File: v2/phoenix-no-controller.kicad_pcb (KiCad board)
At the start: 2 copper layers, 121.5 x 110.3 mm, 66 parts

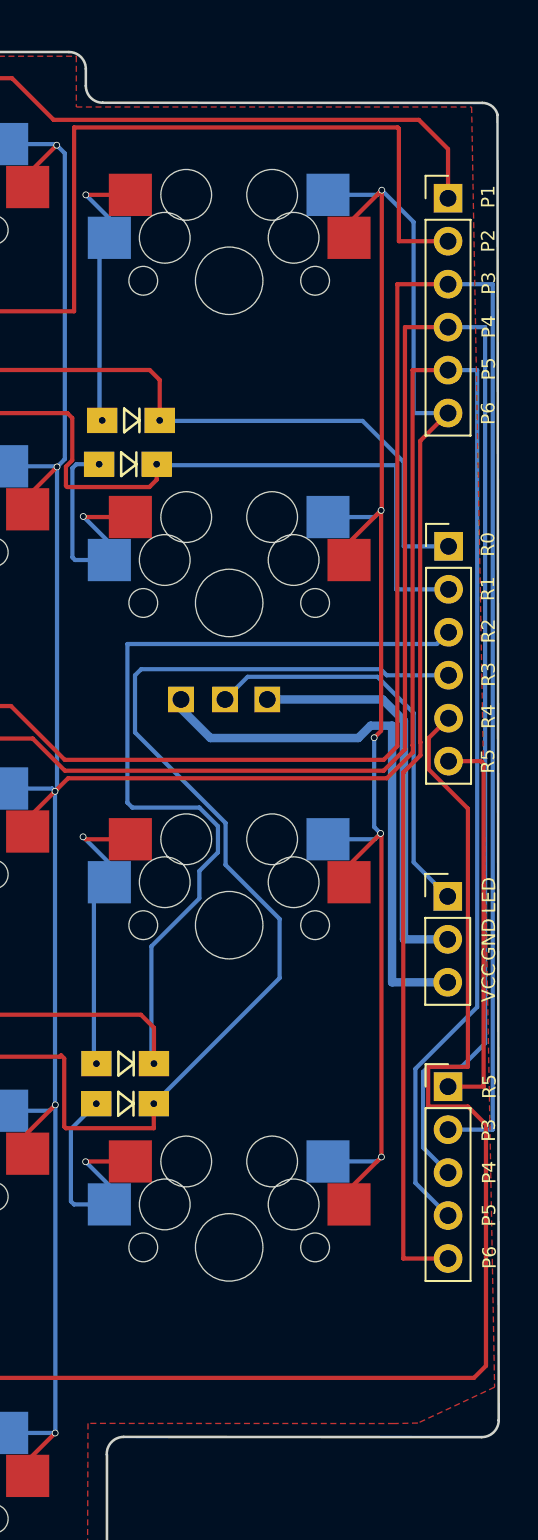
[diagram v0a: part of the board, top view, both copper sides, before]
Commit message: thumb
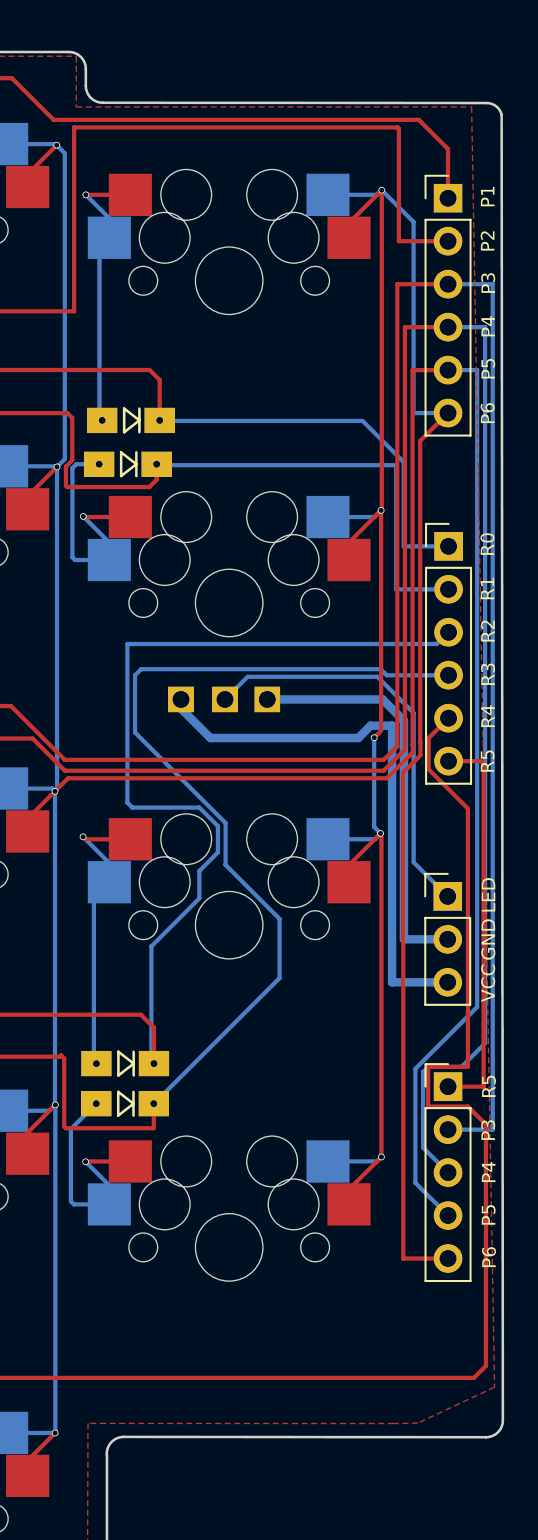
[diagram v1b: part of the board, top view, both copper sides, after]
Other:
- board size 121.5 x 110.3 mm -> 121.8 x 110.3 mm
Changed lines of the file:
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@@
   (gr_arc (start 209.0325 81.84981) (mid 208.325393 81.556917) (end 208.0325 80.84981)
     (stroke (width 0.15) (type solid)) (layer "Edge.Cuts"))
-  (gr_arc (start 250.47 84.86) (mid 251.03946 85.049183) (end 251.37 85.55)
+  (gr_arc (start 250.717102 84.867102) (mid 251.286538 85.056304) (end 251.617102 85.557102)
     (stroke (width 0.15) (type solid)) (layer "Edge.Cuts"))
   (gr_line (start 185.9825 81.84981) (end 168.9825 81.84981)
@@
   (gr_arc (start 186.9825 79.84981) (mid 187.275393 79.142703) (end 187.9825 78.84981)
     (stroke (width 0.15) (type solid)) (layer "Edge.Cuts"))
-  (gr_arc (start 251.442898 162.742898) (mid 251.15 163.45) (end 250.442898 163.742898)
+  (gr_arc (start 251.69 162.75) (mid 251.397107 163.457107) (end 250.69 163.75)
     (stroke (width 0.15) (type solid)) (layer "Edge.Cuts"))
   (gr_line (start 208.0325 80.84981) (end 208.0325 79.84981)
@@
   (gr_arc (start 189.0325 178.09981) (mid 188.739607 178.806917) (end 188.0325 179.09981)
     (stroke (width 0.15) (type solid)) (layer "Edge.Cuts"))
-  (gr_line (start 229.27 163.73) (end 250.442898 163.742898)
+  (gr_line (start 229.27 163.73) (end 250.69 163.75)
     (stroke (width 0.15) (type solid)) (layer "Edge.Cuts"))
   (gr_line (start 190.0325 176.09981) (end 204.9825 176.09981)
     (stroke (width 0.15) (type solid)) (layer "Edge.Cuts"))
-  (gr_line (start 251.442898 162.742898) (end 251.37 85.55)
+  (gr_line (start 251.69 162.75) (end 251.617102 85.557102)
     (stroke (width 0.15) (type solid)) (layer "Edge.Cuts"))
-  (gr_line (start 250.47 84.86) (end 228.0325 84.84981)
+  (gr_line (start 250.717102 84.867102) (end 228.0325 84.84981)
     (stroke (width 0.15) (type solid)) (layer "Edge.Cuts"))
   (gr_arc (start 228.0325 84.84981) (mid 227.325393 84.556917) (end 227.0325 83.84981)
